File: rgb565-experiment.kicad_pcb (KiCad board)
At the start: 4 copper layers, 101.6 x 71.1 mm, 34 parts, among them J1 ST_SHIFTER_SOCKET, J2 Conn_01x02, SW1 SW_SPDT, U1 74HC00, U2 ST_SHIFTER, U3 ST_SHIFTER, U4 74HC245, U5 74LS257, U6 74HC245

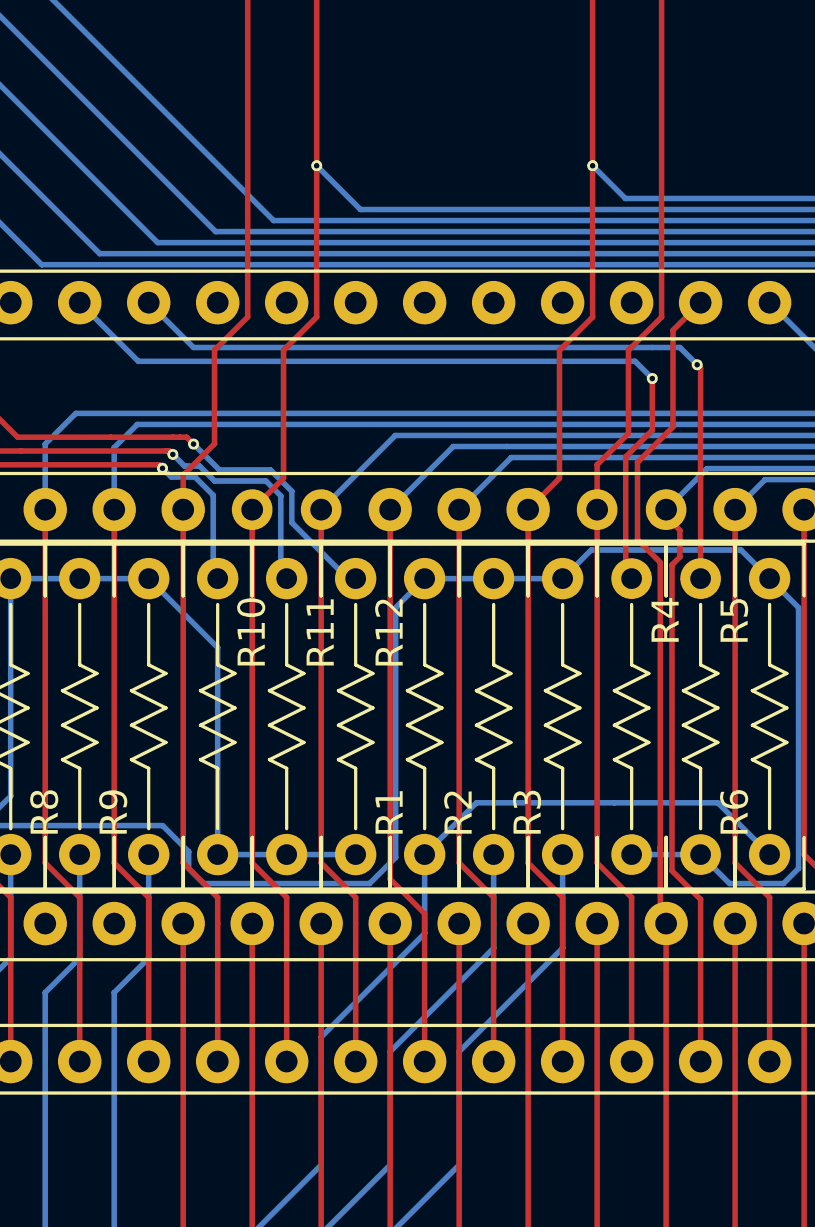
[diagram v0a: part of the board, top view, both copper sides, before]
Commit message: done initial routing
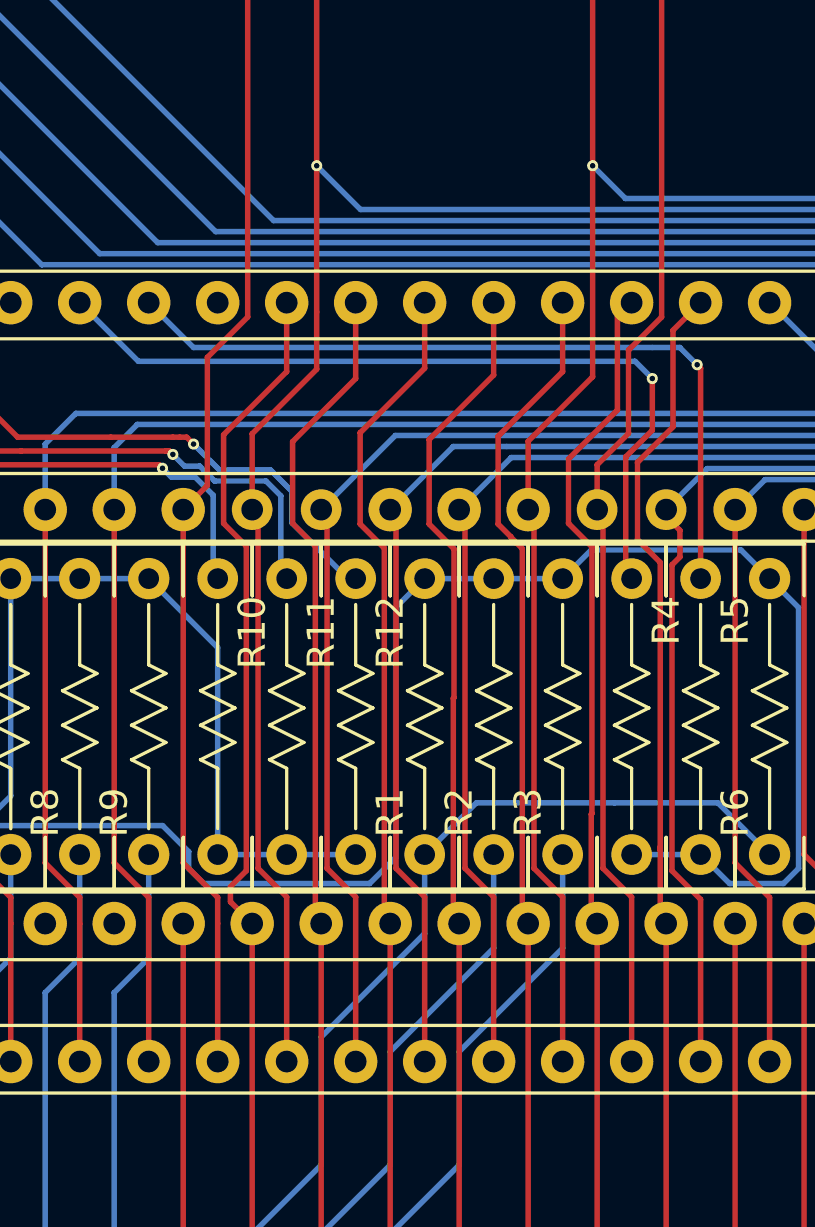
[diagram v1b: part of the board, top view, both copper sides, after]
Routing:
- net /rxw: track 74.8 -> 99.5 mm
- net /a3: track 20.8 -> 45.2 mm
- net /a2: track 20.8 -> 45.1 mm
- net /a4: track 20.8 -> 45.1 mm
- net /a1: track 20.8 -> 45.1 mm
- net /a5: track 96.5 -> 120.7 mm
